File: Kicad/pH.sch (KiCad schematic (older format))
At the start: 5 parts, among them U1 MCP6241

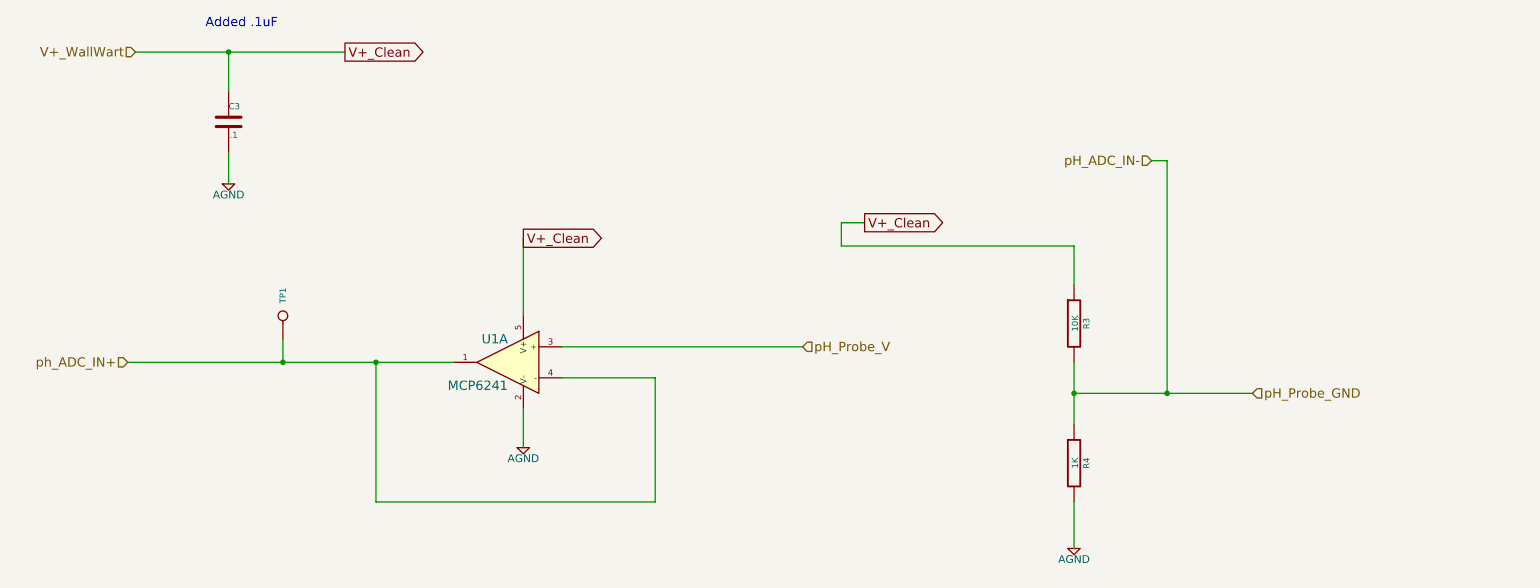
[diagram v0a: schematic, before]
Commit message: updated based on feedback. Ready for second review
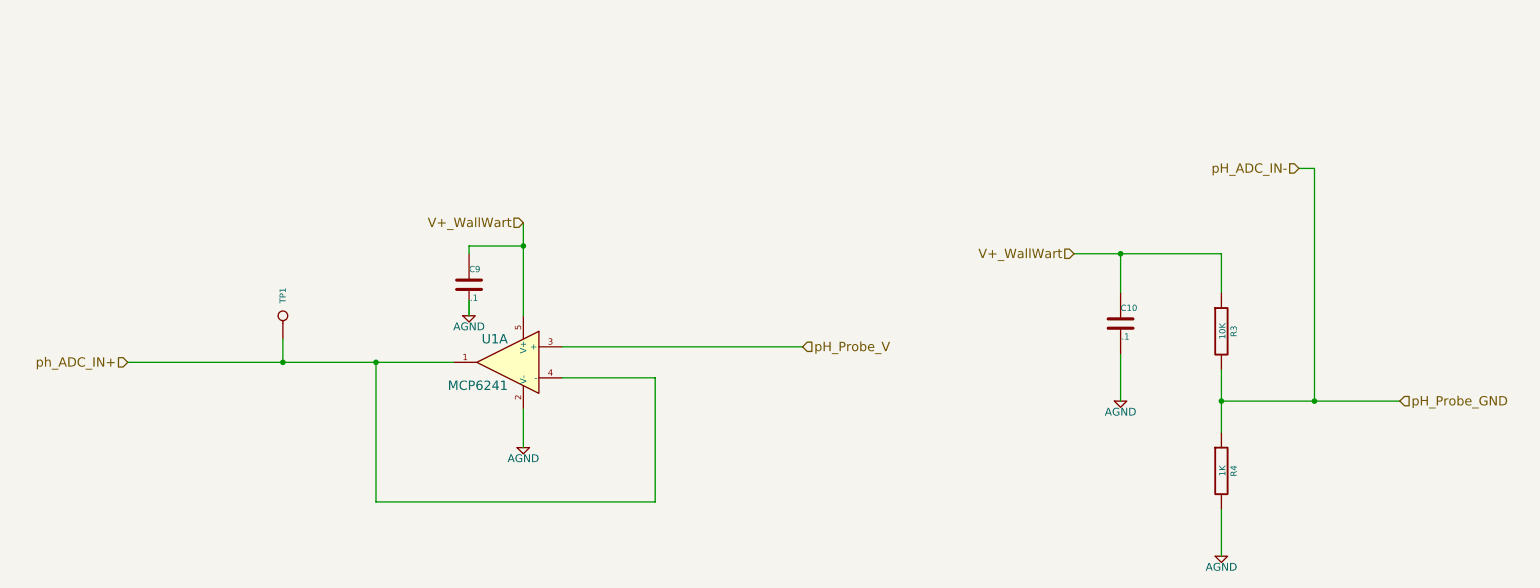
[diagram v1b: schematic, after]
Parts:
- removed C3: .1, ~, symbol C
- added C10, C9: .1, ~, symbol C
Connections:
- net labels removed: V+_Clean
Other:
- note removed: "Added .1uF"
- moved on the sheet: R3, R4
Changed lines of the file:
@@
 Sheet 6 7
 Title ""
-Date "18 oct 2014"
+Date "21 oct 2014"
 Rev ""
 Comp ""
@@
 Comment4 ""
 $EndDescr
-Text HLabel 1400 1200 0    60   Input ~ 0
-V+_WallWart
 Text HLabel 1350 3200 0    60   Input ~ 0
 ph_ADC_IN+
-Wire Wire Line
-	3900 3500 3900 3750
 $Comp
 L R R4
 U 1 1 53D7D158
-P 7450 3850
-F 0 "R4" V 7530 3850 40  0000 C CNN
-F 1 "1K" V 7457 3851 40  0000 C CNN
-F 2 "~" V 7380 3850 30  0000 C CNN
-F 3 "~" H 7450 3850 30  0000 C CNN
-	1    7450 3850
+P 8400 3900
+F 0 "R4" V 8480 3900 40  0000 C CNN
+F 1 "1K" V 8407 3901 40  0000 C CNN
+F 2 "~" V 8330 3900 30  0000 C CNN
+F 3 "~" H 8400 3900 30  0000 C CNN
+	1    8400 3900
 	1    0    0    -1
 $EndComp
-Wire Wire Line
-	1350 3200 3450 3200
-Text HLabel 7950 1900 0    60   Input ~ 0
+Text HLabel 8900 1950 0    60   Input ~ 0
 pH_ADC_IN-
 $Comp
-L AGND #PWR07
+L AGND #PWR08
 U 1 1 53DCC7DA
 P 3900 3750
-F 0 "#PWR07" H 3900 3750 40  0001 C CNN
+F 0 "#PWR08" H 3900 3750 40  0001 C CNN
 F 1 "AGND" H 3900 3680 50  0000 C CNN
 F 2 "" H 3900 3750 60  0000 C CNN
@@
 L R R3
 U 1 1 53F37946
-P 7450 2950
-F 0 "R3" V 7530 2950 40  0000 C CNN
-F 1 "10K" V 7457 2951 40  0000 C CNN
-F 2 "~" V 7380 2950 30  0000 C CNN
-F 3 "~" H 7450 2950 30  0000 C CNN
-	1    7450 2950
+P 8400 3000
+F 0 "R3" V 8480 3000 40  0000 C CNN
+F 1 "10K" V 8407 3001 40  0000 C CNN
+F 2 "~" V 8330 3000 30  0000 C CNN
+F 3 "~" H 8400 3000 30  0000 C CNN
+	1    8400 3000
 	1    0    0    -1
 $EndComp
@@
 	0    -1   -1   0
 $EndComp
+Text HLabel 5700 3100 2    60   Input ~ 0
+pH_Probe_V
+$Comp
+L AGND #PWR09
+U 1 1 540C92AB
+P 8400 4450
+F 0 "#PWR09" H 8400 4450 40  0001 C CNN
+F 1 "AGND" H 8400 4380 50  0000 C CNN
+F 2 "" H 8400 4450 60  0000 C CNN
+F 3 "" H 8400 4450 60  0000 C CNN
+	1    8400 4450
+	1    0    0    -1
+$EndComp
+Text HLabel 9550 3450 2    60   Input ~ 0
+pH_Probe_GND
+$Comp
+L C C9
+U 1 1 54453E50
+P 3550 2700
+F 0 "C9" H 3550 2800 40  0000 L CNN
+F 1 ".1" H 3556 2615 40  0000 L CNN
+F 2 "~" H 3588 2550 30  0000 C CNN
+F 3 "~" H 3550 2700 60  0000 C CNN
+	1    3550 2700
+	1    0    0    -1
+$EndComp
+Text HLabel 3900 2300 0    60   Input ~ 0
+V+_WallWart
+$Comp
+L AGND #PWR010
+U 1 1 54453F29
+P 3550 2900
+F 0 "#PWR010" H 3550 2900 40  0001 C CNN
+F 1 "AGND" H 3550 2830 50  0000 C CNN
+F 2 "" H 3550 2900 60  0000 C CNN
+F 3 "" H 3550 2900 60  0000 C CNN
+	1    3550 2900
+	1    0    0    -1
+$EndComp
+Wire Wire Line
+	3900 3500 3900 3750
+Wire Wire Line
+	1350 3200 3450 3200
 Wire Wire Line
 	2350 3050 2350 3200
 Connection ~ 2350 3200
 Wire Wire Line
-	7450 3200 7450 3600
-Text HLabel 5700 3100 2    60   Input ~ 0
-pH_Probe_V
+	8400 3250 8400 3650
 Wire Wire Line
 	4150 3100 5700 3100
@@
 	4750 3300 4150 3300
 Connection ~ 2950 3200
+Wire Wire Line
+	8400 4450 8400 4150
+Wire Wire Line
+	9000 1950 9000 3450
+Wire Wire Line
+	9000 1950 8900 1950
+Wire Wire Line
+	8400 3450 9550 3450
+Connection ~ 8400 3450
+Connection ~ 9000 3450
+Wire Wire Line
+	3900 2300 3900 2900
+Wire Wire Line
+	8400 2500 8400 2750
+Wire Wire Line
+	3550 2500 3550 2450
+Wire Wire Line
+	3550 2450 3900 2450
+Connection ~ 3900 2450
+Wire Wire Line
+	3550 2800 3550 2900
 $Comp
-L AGND #PWR08
-U 1 1 540C92AB
-P 7450 4400
-F 0 "#PWR08" H 7450 4400 40  0001 C CNN
-F 1 "AGND" H 7450 4330 50  0000 C CNN
-F 2 "" H 7450 4400 60  0000 C CNN
-F 3 "" H 7450 4400 60  0000 C CNN
-	1    7450 4400
+L C C10
+U 1 1 54453F94
+P 7750 2950
+F 0 "C10" H 7750 3050 40  0000 L CNN
+F 1 ".1" H 7756 2865 40  0000 L CNN
+F 2 "~" H 7788 2800 30  0000 C CNN
+F 3 "~" H 7750 2950 60  0000 C CNN
+	1    7750 2950
 	1    0    0    -1
 $EndComp
 Wire Wire Line
-	7450 4400 7450 4100
-Text HLabel 8600 3400 2    60   Input ~ 0
-pH_Probe_GND
-Wire Wire Line
-	8050 1900 8050 3400
-Wire Wire Line
-	8050 1900 7950 1900
-Wire Wire Line
-	7450 3400 8600 3400
-Connection ~ 7450 3400
-Connection ~ 8050 3400
+	7750 2750 7750 2500
 $Comp
-L C C3
-U 1 1 5441038F
-P 2000 1650
-F 0 "C3" H 2000 1750 40  0000 L CNN
-F 1 ".1" H 2006 1565 40  0000 L CNN
-F 2 "~" H 2038 1500 30  0000 C CNN
-F 3 "~" H 2000 1650 60  0000 C CNN
-	1    2000 1650
+L AGND #PWR011
+U 1 1 54453FBC
+P 7750 3450
+F 0 "#PWR011" H 7750 3450 40  0001 C CNN
+F 1 "AGND" H 7750 3380 50  0000 C CNN
+F 2 "" H 7750 3450 60  0000 C CNN
+F 3 "" H 7750 3450 60  0000 C CNN
+	1    7750 3450
 	1    0    0    -1
 $EndComp
 Wire Wire Line
-	5950 2450 7450 2450
-Text Notes 1850 1050 0    60   ~ 0
-Added .1uF
+	7750 3450 7750 3150
+Text HLabel 7450 2500 0    60   Input ~ 0
+V+_WallWart
 Wire Wire Line
-	1400 1200 2750 1200
-Wire Wire Line
-	2000 1450 2000 1200
-Connection ~ 2000 1200
-$Comp
-L AGND #PWR09
-U 1 1 5441062F
-P 2000 2050
-F 0 "#PWR09" H 2000 2050 40  0001 C CNN
-F 1 "AGND" H 2000 1980 50  0000 C CNN
-F 2 "" H 2000 2050 60  0000 C CNN
-F 3 "" H 2000 2050 60  0000 C CNN
-	1    2000 2050
-	1    0    0    -1
-$EndComp
-Wire Wire Line
-	2000 1850 2000 2050
-Wire Wire Line
-	3900 2900 3900 2400
-Wire Wire Line
-	7450 2450 7450 2700
-Text GLabel 2750 1200 2    60   Output ~ 0
-V+_Clean
-Text GLabel 3900 2400 2    60   Output ~ 0
-V+_Clean
-Text GLabel 6100 2300 2    60   Output ~ 0
-V+_Clean
-Wire Wire Line
-	5950 2450 5950 2300
-Wire Wire Line
-	5950 2300 6100 2300
+	7450 2500 8400 2500
+Connection ~ 7750 2500
 $EndSCHEMATC
